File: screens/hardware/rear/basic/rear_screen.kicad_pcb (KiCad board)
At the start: 2 copper layers, 112 x 79.4 mm, 46 parts, among them J1 Conn_01x02_Pin, J13 USB_C_Receptacle_USB2.0, J2 Conn_01x02_Pin, J3 Conn_01x02_Pin, J4 Conn_01x02_Pin, J5 Conn_01x02_Pin, J6 Conn_01x02_Pin, J7 Conn_01x08_Socket, Q1 NTMFS4C03N-HXY, Q2 NTMFS4C03N-HXY, Q3 NTMFS4C03N-HXY, Q4 NTMFS4C03N-HXY, Q6 NTMFS4C03N-HXY, Q7 NTMFS4C03N-HXY, U1 MIC4426, U2 MIC4426, U3 AOZ1280CI

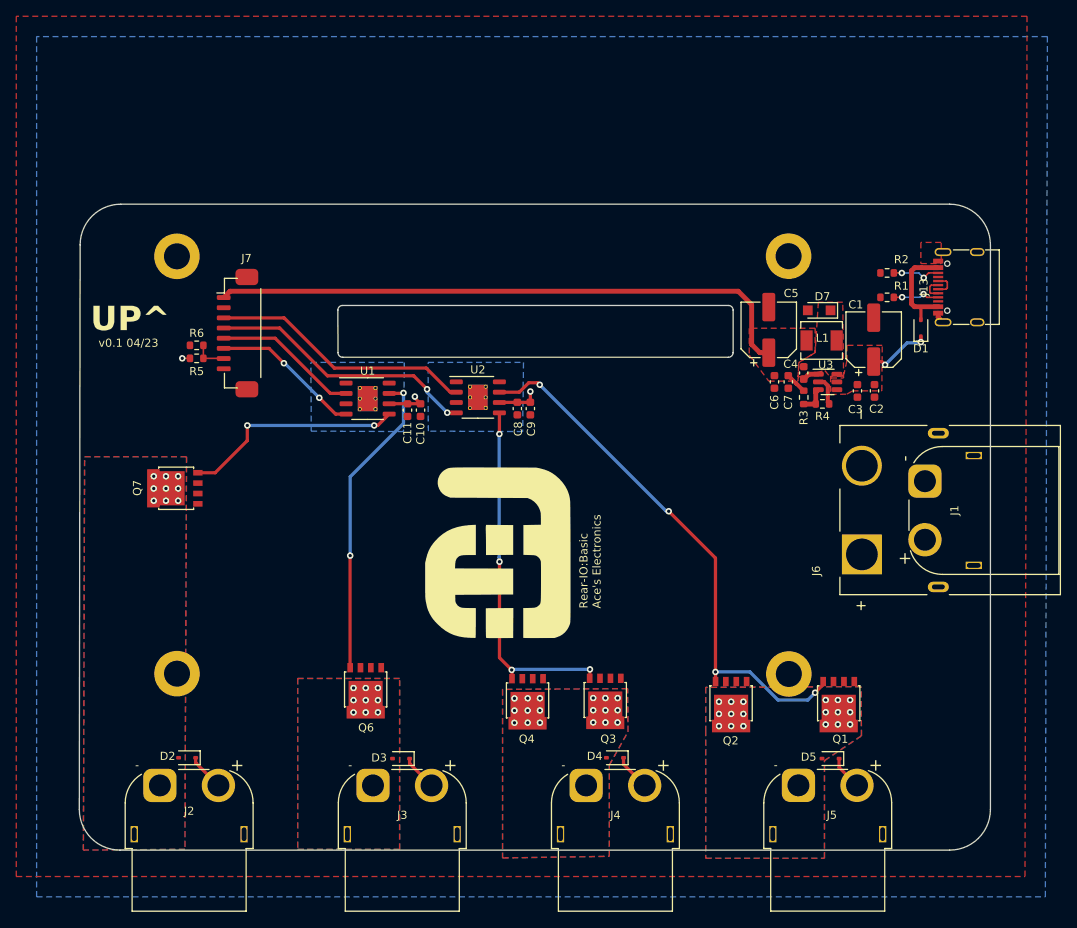
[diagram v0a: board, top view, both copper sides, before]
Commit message: Sent to JLCPCB as Rev0
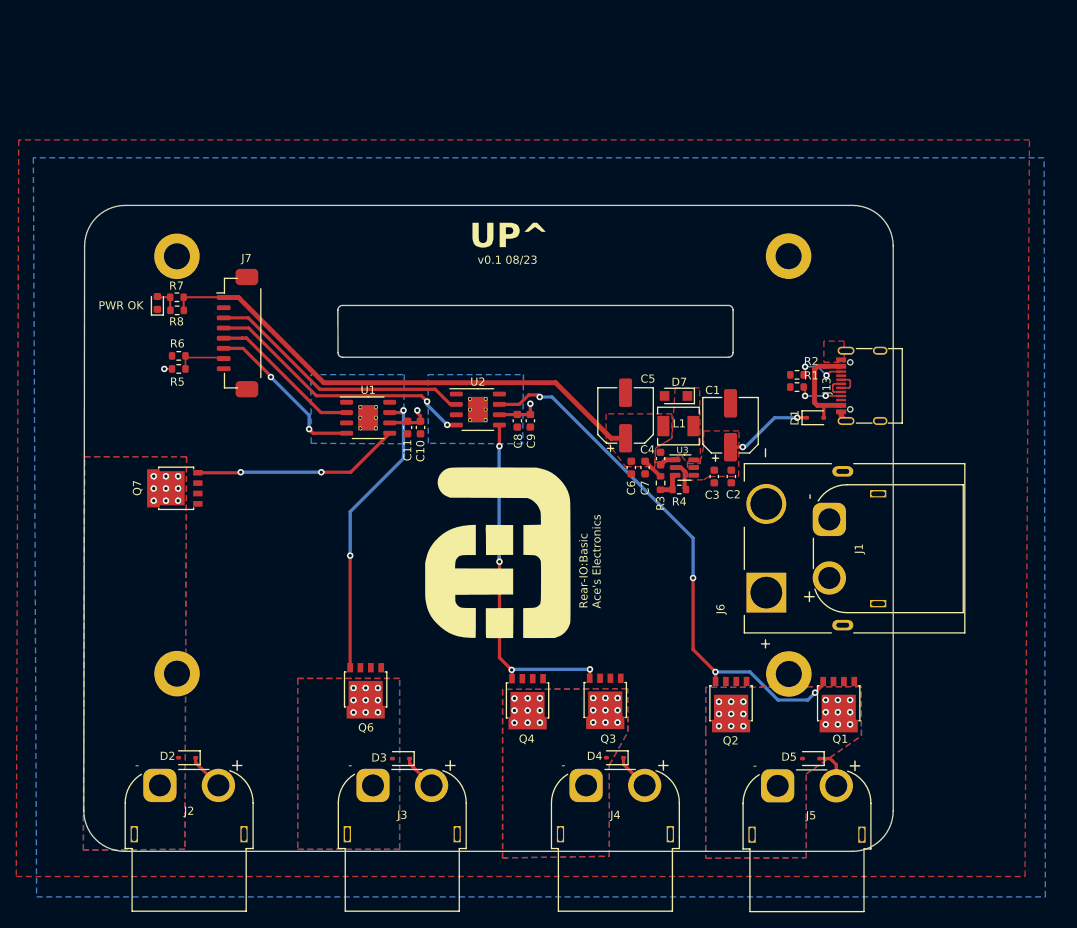
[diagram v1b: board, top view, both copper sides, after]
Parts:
- added D6: LED_Small, LED_SMD:LED_0603_1608Metric, F.Cu at (87.8, 73.7)
- added R7: 5.1k, Resistor_SMD:R_0603_1608Metric, F.Cu at (90.2, 73.0)
- added R8: 5.1k, Resistor_SMD:R_0603_1608Metric, F.Cu at (90.2, 74.6)
- moved C1 20.5 mm to (158.2, 88.7)
- moved R3 20.5 mm to (149.6, 95.8)
- moved R4 20.5 mm to (151.9, 96.6)
- moved C3 20.5 mm to (156.2, 95.0)
- moved C7 20.5 mm to (147.7, 93.9)
- moved C2 20.5 mm to (158.3, 95.0)
- moved C4 20.5 mm to (149.6, 92.8)
- moved C5 20.5 mm to (145.3, 87.5)
- moved D7 20.5 mm to (151.5, 85.1)
- moved L1 20.5 mm to (151.8, 88.8)
- moved C6 20.5 mm to (146.0, 93.9)
- moved U3 20.5 mm to (152.5, 93.9)
- moved D1 17.0 mm to (168.6, 87.8), turned to 0 degrees
- moved J13 17.0 mm to (175.5, 83.9)
- moved R2 16.7 mm to (166.4, 82.5)
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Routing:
- net +5V: track 76.0 -> 65.8 mm
- net VIN: track 36.5 -> 40.8 mm
- net Net-(D6-A): track 0.00 -> 3.23 mm
- net GPIO14: track 4.11 -> 6.41 mm
- net Net-(Q6-G): track 38.3 -> 36.2 mm
- net GPIO13: track 18.4 -> 20.5 mm
- net Net-(Q7-G): track 27.6 -> 25.6 mm
- net Net-(Q3-G): track 44.1 -> 42.6 mm
- net GPIO12: track 17.9 -> 18.9 mm
- net Net-(Q1-G): track 67.0 -> 66.2 mm
- net GPIO11: track 33.1 -> 33.8 mm
- net GPIO10: track 32.4 -> 33.0 mm
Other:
- board size 112 x 79.4 mm -> 99.5 x 79.4 mm
- board text added: "PWR OK"
- board text added: "v0.1 08/23"
- board text removed: "v0.1 04/23"
